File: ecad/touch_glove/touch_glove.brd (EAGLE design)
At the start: 78.3 x 40.6 mm, 177 parts, among them Q1 MCH3474 4A/30V, Q2 MCH3474 4A/30V, Q3 MCH3474 4A/30V, Q4 MCH3474 4A/30V, Q5 MCH3474 4A/30V, Q6 MCH3474 4A/30V, SW1 4A/28V

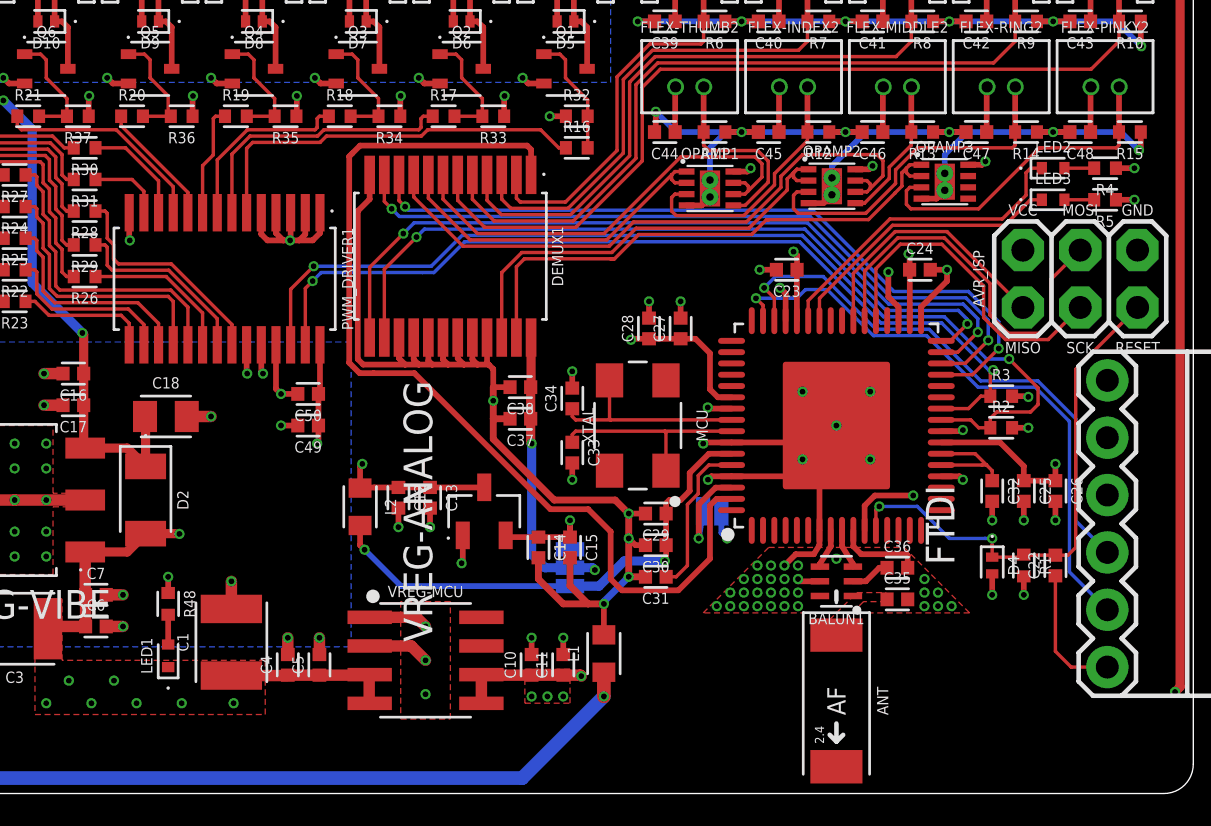
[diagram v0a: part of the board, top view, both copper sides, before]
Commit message: Add several test codes for PCB.
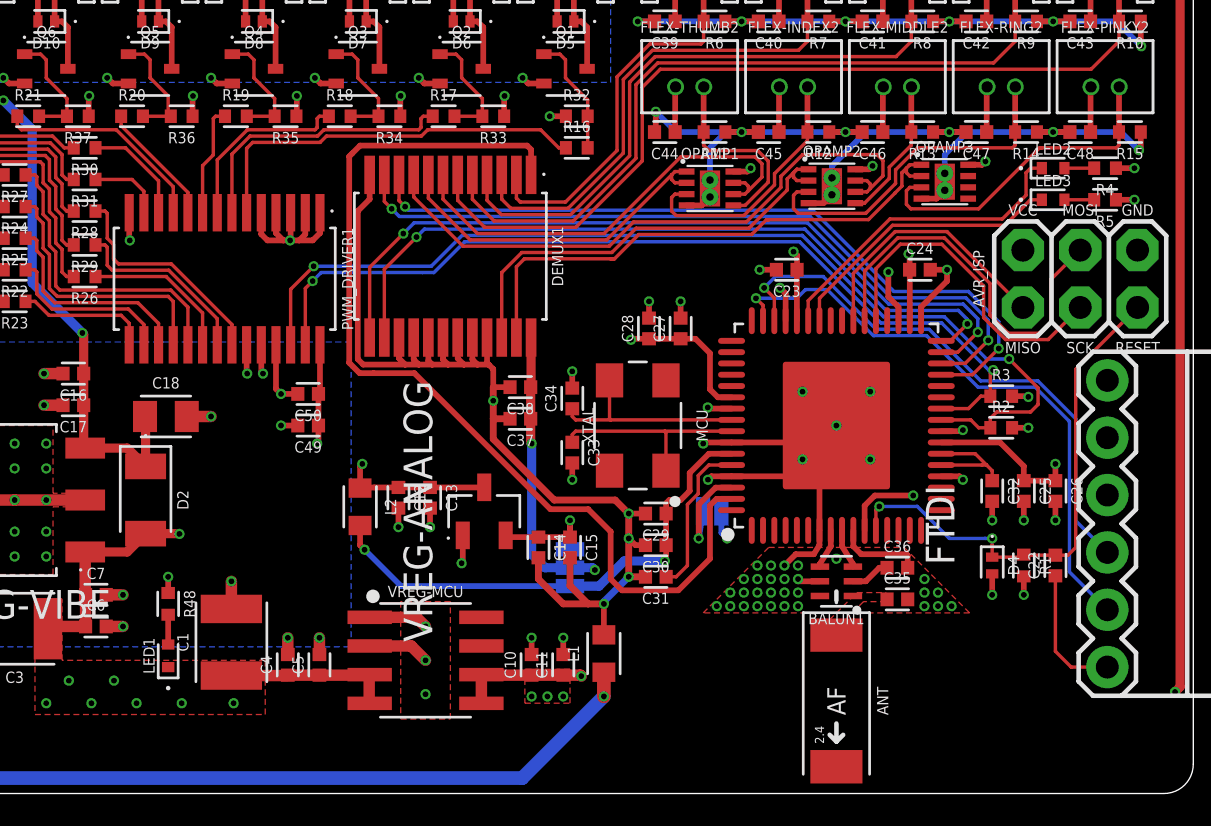
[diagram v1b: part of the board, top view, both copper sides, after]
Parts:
- LIPO1: value Molex RA 2mm pitch -> 7.4V
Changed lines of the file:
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@@
 <?xml version="1.0" encoding="utf-8"?>
 <!DOCTYPE eagle SYSTEM "eagle.dtd">
-<eagle version="9.1.0">
+<eagle version="9.1.3">
 <drawing>
 <settings>
@@
 <attribute name="MFR" value="Comchip Technology" x="31.9" y="13" size="1.778" layer="27" rot="R270" display="off"/>
 <attribute name="MPN" value="CGRKM4001-HF" x="31.9" y="13" size="1.778" layer="27" rot="R270" display="off"/>
+<attribute name="VALUE" value="1A/50V" x="31.9" y="13" size="1.778" layer="27" rot="R270" display="off"/>
 </element>
 <element name="D3" library="PiB_discrete_semiconductors" package="SODFL3516X170" package3d_urn="urn:adsk.eagle:package:2939213/1" value="1A/50V" x="20" y="19.8" rot="R270">
@@
 <attribute name="MFR" value="Comchip Technology" x="20" y="19.8" size="1.778" layer="27" rot="R270" display="off"/>
 <attribute name="MPN" value="CGRKM4001-HF" x="20" y="19.8" size="1.778" layer="27" rot="R270" display="off"/>
+<attribute name="VALUE" value="1A/50V" x="20" y="19.8" size="1.778" layer="27" rot="R270" display="off"/>
 </element>
 <element name="D6" library="PiB_discrete_semiconductors" package="DFN100X60X55-2" package3d_urn="urn:adsk.eagle:package:2933421/1" value="150mA/75V" x="45.9" y="34.2" rot="R180">
@@
 <attribute name="VALUE" value="250mA/3.3V" x="46.9" y="12.5" size="1.778" layer="27" rot="R90" display="off"/>
 </element>
-<element name="LIPO1" library="PiB_batteries" package="BATTERY_MOLEX-89401_RA_PITCH-2MM" package3d_urn="urn:adsk.eagle:package:2971487/3" value="Molex RA 2mm pitch" x="19.2" y="6.7" rot="R180">
+<element name="LIPO1" library="PiB_batteries" package="BATTERY_MOLEX-89401_RA_PITCH-2MM" package3d_urn="urn:adsk.eagle:package:2971487/3" value="7.4V" x="19.2" y="6.7" rot="R180">
 <attribute name="DATASHEET" value="https://www.molex.com/pdm_docs/sd/894010210_sd.pdf" x="19.2" y="6.7" size="1.778" layer="27" font="vector" rot="R180" display="off"/>
 <attribute name="DATASHEET_CONNECTOR" value="https://www.molex.com/pdm_docs/sd/873690200_sd.pdf" x="19.2" y="6.7" size="1.778" layer="27" font="vector" rot="R180" display="off"/>
